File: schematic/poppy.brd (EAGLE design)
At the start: 31 x 51.9 mm, 18 parts, among them Q1 8MHz, U1 ATMEGA16U4TQFP44, U2 MBI5030GFSOP-24

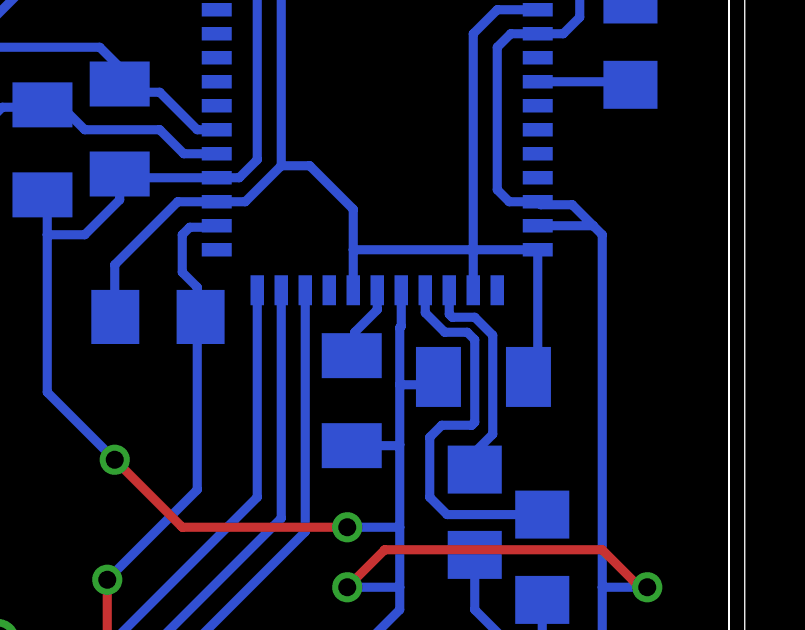
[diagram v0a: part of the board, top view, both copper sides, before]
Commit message: printed
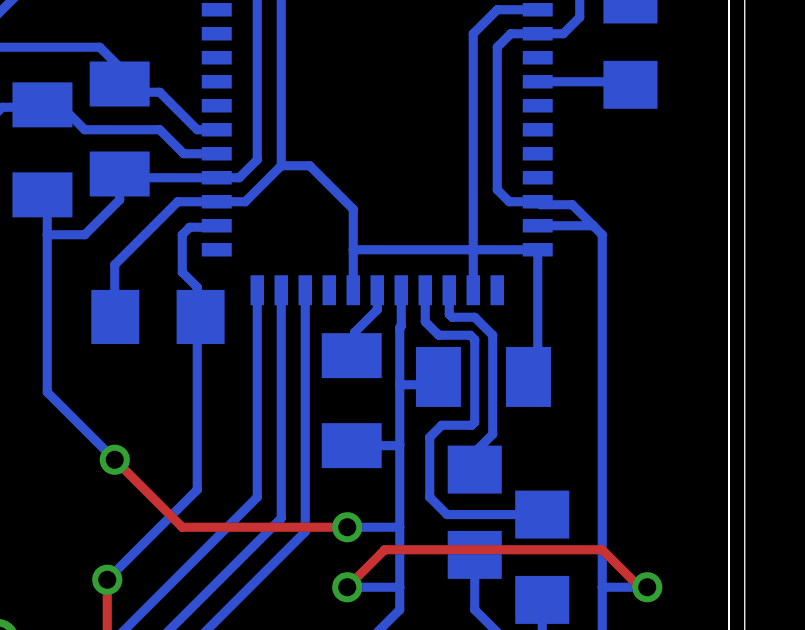
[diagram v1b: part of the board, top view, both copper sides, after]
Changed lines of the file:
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@@
 <grid distance="0.25" unitdist="mm" unit="mm" style="lines" multiple="1" display="no" altdistance="0.1" altunitdist="mm" altunit="mm"/>
 <layers>
-<layer number="1" name="Top" color="4" fill="1" visible="yes" active="yes"/>
+<layer number="1" name="Top" color="4" fill="1" visible="no" active="yes"/>
 <layer number="16" name="Bottom" color="1" fill="1" visible="yes" active="yes"/>
 <layer number="17" name="Pads" color="2" fill="1" visible="yes" active="yes"/>
@@
 <layer number="19" name="Unrouted" color="6" fill="1" visible="yes" active="yes"/>
 <layer number="20" name="Dimension" color="15" fill="1" visible="yes" active="yes"/>
-<layer number="21" name="tPlace" color="7" fill="1" visible="yes" active="yes"/>
-<layer number="22" name="bPlace" color="7" fill="1" visible="yes" active="yes"/>
-<layer number="23" name="tOrigins" color="15" fill="1" visible="yes" active="yes"/>
-<layer number="24" name="bOrigins" color="15" fill="1" visible="yes" active="yes"/>
-<layer number="25" name="tNames" color="7" fill="1" visible="yes" active="yes"/>
-<layer number="26" name="bNames" color="7" fill="1" visible="yes" active="yes"/>
+<layer number="21" name="tPlace" color="7" fill="1" visible="no" active="yes"/>
+<layer number="22" name="bPlace" color="7" fill="1" visible="no" active="yes"/>
+<layer number="23" name="tOrigins" color="15" fill="1" visible="no" active="yes"/>
+<layer number="24" name="bOrigins" color="15" fill="1" visible="no" active="yes"/>
+<layer number="25" name="tNames" color="7" fill="1" visible="no" active="yes"/>
+<layer number="26" name="bNames" color="7" fill="1" visible="no" active="yes"/>
 <layer number="27" name="tValues" color="7" fill="1" visible="no" active="yes"/>
 <layer number="28" name="bValues" color="7" fill="1" visible="no" active="yes"/>
-<layer number="29" name="tStop" color="7" fill="3" visible="yes" active="yes"/>
-<layer number="30" name="bStop" color="7" fill="6" visible="yes" active="yes"/>
+<layer number="29" name="tStop" color="7" fill="3" visible="no" active="yes"/>
+<layer number="30" name="bStop" color="7" fill="6" visible="no" active="yes"/>
 <layer number="31" name="tCream" color="7" fill="4" visible="no" active="yes"/>
 <layer number="32" name="bCream" color="7" fill="5" visible="no" active="yes"/>
 <layer number="33" name="tFinish" color="6" fill="3" visible="yes" active="yes"/>
 <layer number="34" name="bFinish" color="6" fill="6" visible="yes" active="yes"/>
-<layer number="35" name="tGlue" color="7" fill="4" visible="yes" active="yes"/>
+<layer number="35" name="tGlue" color="7" fill="4" visible="no" active="yes"/>
 <layer number="36" name="bGlue" color="7" fill="5" visible="no" active="yes"/>
-<layer number="37" name="tTest" color="7" fill="1" visible="yes" active="yes"/>
-<layer number="38" name="bTest" color="7" fill="1" visible="yes" active="yes"/>
+<layer number="37" name="tTest" color="7" fill="1" visible="no" active="yes"/>
+<layer number="38" name="bTest" color="7" fill="1" visible="no" active="yes"/>
 <layer number="39" name="tKeepout" color="4" fill="11" visible="no" active="yes"/>
 <layer number="40" name="bKeepout" color="1" fill="11" visible="no" active="yes"/>
@@
 <layer number="42" name="bRestrict" color="1" fill="10" visible="no" active="yes"/>
 <layer number="43" name="vRestrict" color="2" fill="10" visible="no" active="yes"/>
-<layer number="44" name="Drills" color="7" fill="1" visible="yes" active="yes"/>
-<layer number="45" name="Holes" color="7" fill="1" visible="yes" active="yes"/>
+<layer number="44" name="Drills" color="7" fill="1" visible="no" active="yes"/>
+<layer number="45" name="Holes" color="7" fill="1" visible="no" active="yes"/>
 <layer number="46" name="Milling" color="3" fill="1" visible="yes" active="yes"/>
-<layer number="47" name="Measures" color="7" fill="1" visible="yes" active="yes"/>
-<layer number="48" name="Document" color="7" fill="1" visible="yes" active="yes"/>
-<layer number="49" name="Reference" color="7" fill="1" visible="yes" active="yes"/>
+<layer number="47" name="Measures" color="7" fill="1" visible="no" active="yes"/>
+<layer number="48" name="Document" color="7" fill="1" visible="no" active="yes"/>
+<layer number="49" name="Reference" color="7" fill="1" visible="no" active="yes"/>
 <layer number="50" name="dxf" color="7" fill="1" visible="no" active="no"/>
-<layer number="51" name="tDocu" color="7" fill="1" visible="yes" active="yes"/>
-<layer number="52" name="bDocu" color="7" fill="1" visible="yes" active="yes"/>
+<layer number="51" name="tDocu" color="7" fill="1" visible="no" active="yes"/>
+<layer number="52" name="bDocu" color="7" fill="1" visible="no" active="yes"/>
 <layer number="53" name="tGND_GNDA" color="7" fill="9" visible="no" active="no"/>
 <layer number="54" name="bGND_GNDA" color="1" fill="9" visible="no" active="no"/>
@@
 <contactref element="U1" pad="4"/>
 <contactref element="R1" pad="1"/>
-<wire x1="19.85" y1="24.4" x2="19.85" y2="23.65" width="0.3048" layer="16"/>
-<wire x1="20.5" y1="20.25" x2="19.75" y2="19.5" width="0" layer="19" extent="1-16"/>
-<wire x1="19.75" y1="19.5" x2="19.75" y2="18" width="0" layer="19" extent="1-16"/>
-<wire x1="19.75" y1="18" x2="20.25" y2="17.5" width="0" layer="19" extent="1-16"/>
-<wire x1="20.25" y1="17.5" x2="23.578" y2="17.5" width="0" layer="19" extent="1-16"/>
-<wire x1="19.85" y1="23.65" x2="20.5" y2="23" width="0.3048" layer="16"/>
-<wire x1="20.5" y1="23" x2="21.25" y2="23" width="0.3048" layer="16"/>
-<wire x1="21.25" y1="23" x2="21.5" y2="22.75" width="0.3048" layer="16"/>
+<wire x1="19.85" y1="24.4" x2="19.85" y2="23.35" width="0.3048" layer="16"/>
 <wire x1="21.5" y1="22.75" x2="21.5" y2="20" width="0.3048" layer="16"/>
-<wire x1="21.5" y1="20.5" x2="21.25" y2="20.25" width="0" layer="19" extent="1-16"/>
-<wire x1="21.25" y1="20.25" x2="20.5" y2="20.25" width="0" layer="19" extent="1-16"/>
 <wire x1="23.75" y1="16.922" x2="20.578" y2="16.922" width="0.3048" layer="16"/>
 <wire x1="20.578" y1="16.922" x2="20" y2="17.5" width="0.3048" layer="16"/>
 <wire x1="20" y1="17.5" x2="20" y2="19.5" width="0.3048" layer="16"/>
 <wire x1="20" y1="19.5" x2="20.4" y2="19.9" width="0.3048" layer="16"/>
-<wire x1="21.5" y1="20.5" x2="21.5" y2="20" width="0" layer="19" extent="1-16"/>
 <wire x1="21.5" y1="20" x2="21.4" y2="19.9" width="0.3048" layer="16"/>
 <wire x1="21.4" y1="19.9" x2="20.4" y2="19.9" width="0.3048" layer="16"/>
+<wire x1="19.85" y1="23.35" x2="20.3" y2="22.9" width="0.3048" layer="16"/>
+<wire x1="20.3" y1="22.9" x2="21.35" y2="22.9" width="0.3048" layer="16"/>
+<wire x1="21.35" y1="22.9" x2="21.5" y2="22.75" width="0.3048" layer="16"/>
 </signal>
 <signal name="N$10">
